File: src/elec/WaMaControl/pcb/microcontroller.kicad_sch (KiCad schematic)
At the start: 6 parts, among them U3 ESP32-S2-WROVER

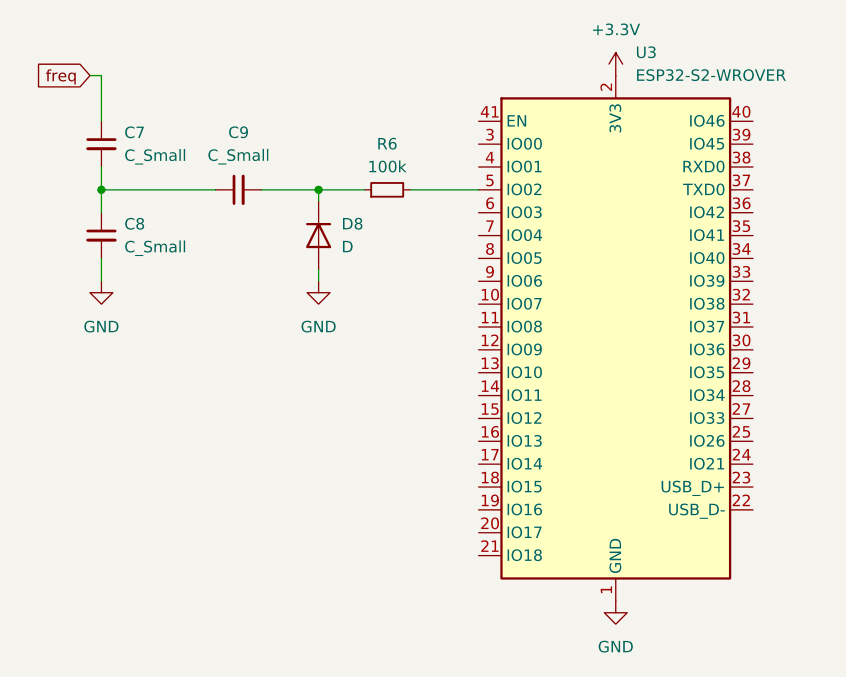
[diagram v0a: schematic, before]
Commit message: - migration of development files from 01-02-25
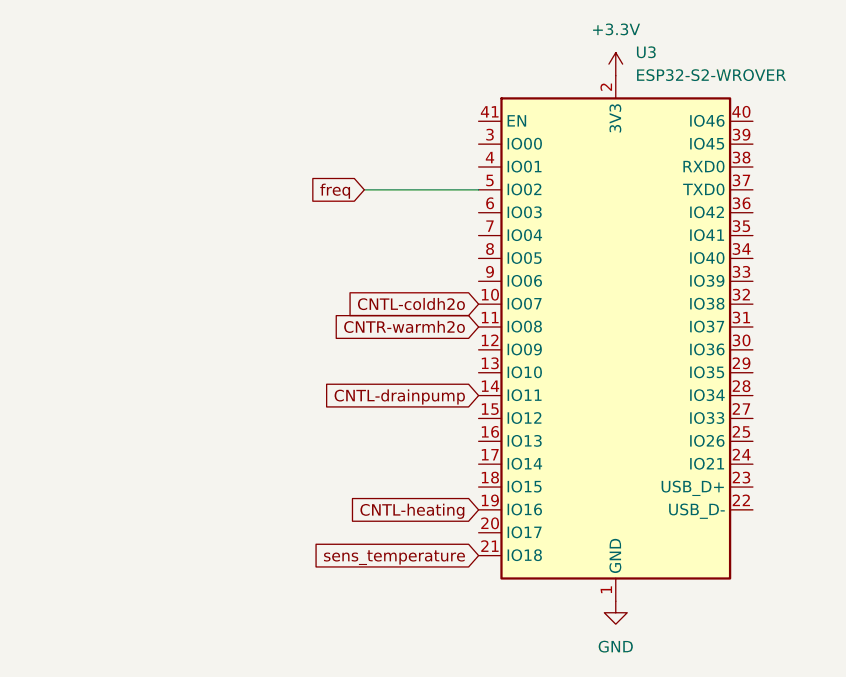
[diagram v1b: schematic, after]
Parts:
- removed C7, C8, C9: C_Small, symbol Device:C_Small
- removed D8: D, symbol Device:D
- removed R6: 100k, symbol Device:R_Small
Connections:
- net freq: now also U3.5 (IO02)
- net CNTL-coldh2o: now reaches U3.10 (IO07)
- net CNTR-warmh2o: now reaches U3.11 (IO08)
- net CNTL-drainpump: now reaches U3.14 (IO11)
- net CNTL-heating: now reaches U3.19 (IO16)
- net sens_temperature: now reaches U3.21 (IO18)
